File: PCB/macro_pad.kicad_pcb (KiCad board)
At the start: 2 copper layers, 112.3 x 92.7 mm, 57 parts, among them J1 OLED, J2 SWD, SW1 SW_Push_45deg, SW10 SW_Push_45deg, SW11 SW_Push_45deg, SW12 SW_Push_45deg, SW13 SW_Push_45deg, SW14 SW_Push_45deg, SW15 SW_Push_45deg, SW16 SW_Push_45deg, SW17 RotaryEncoder_Switch, SW18 RotaryEncoder_Switch, SW2 SW_Push_45deg, SW3 SW_Push_45deg, SW4 SW_Push_45deg, SW5 SW_Push_45deg, SW6 SW_Push_45deg, SW7 SW_Push_45deg, SW8 SW_Push_45deg, SW9 SW_Push_45deg

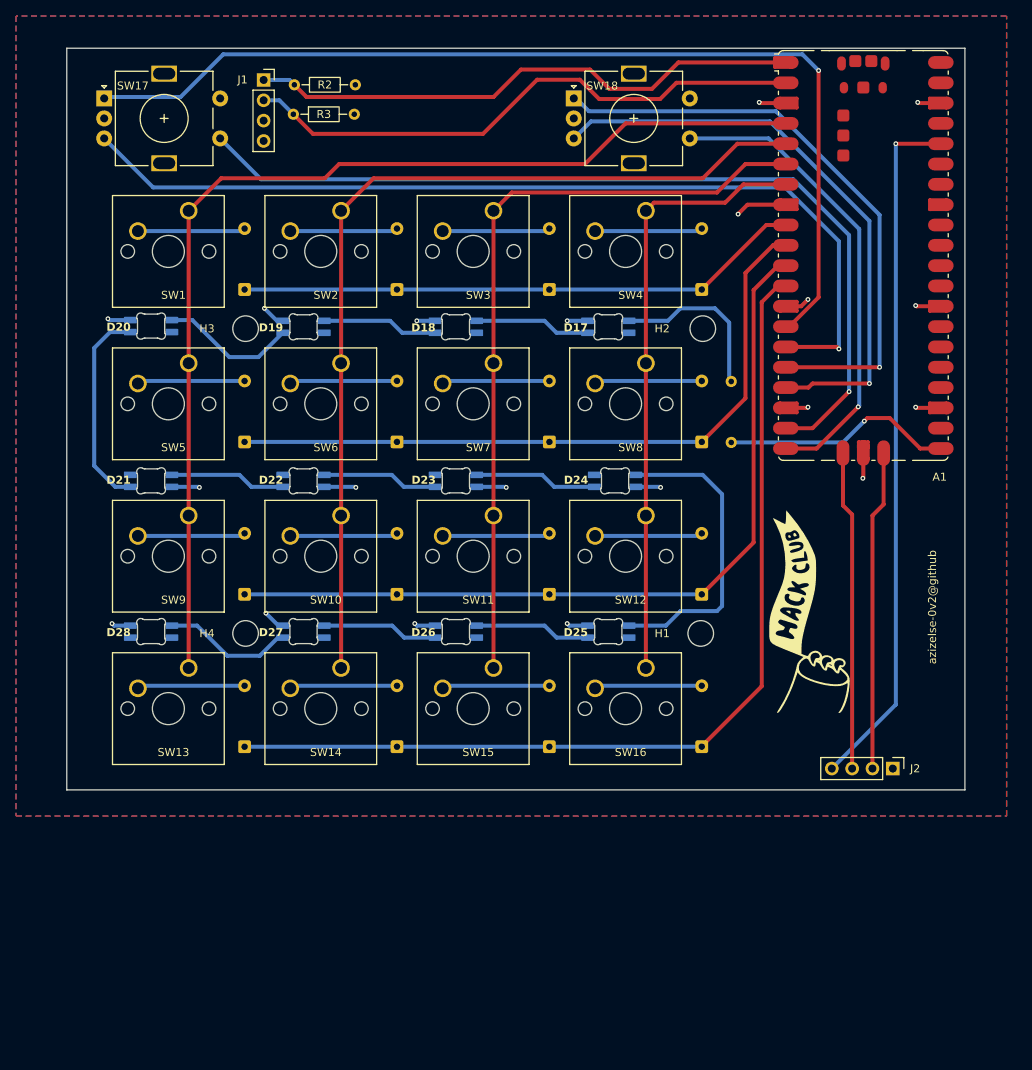
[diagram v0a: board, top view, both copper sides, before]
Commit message: Followed guidelines on schem
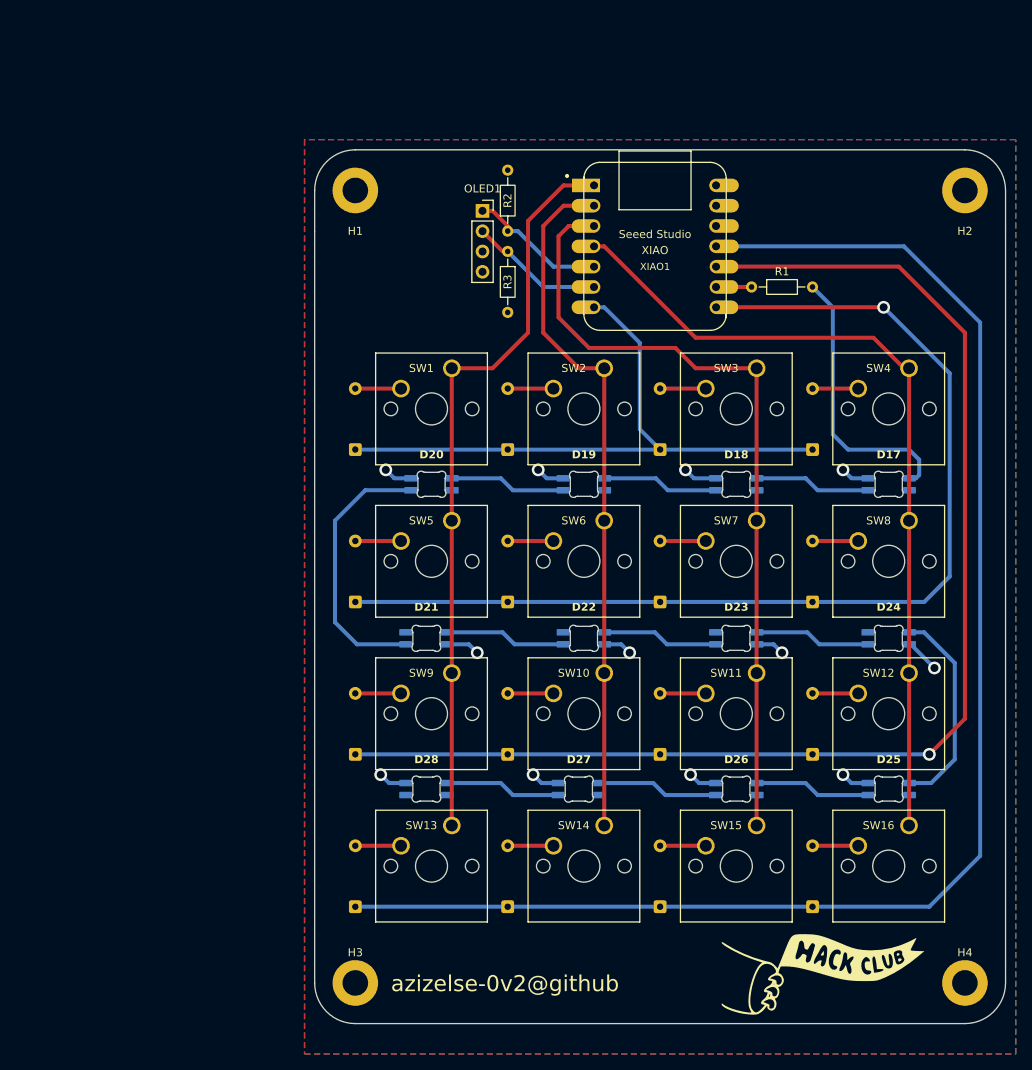
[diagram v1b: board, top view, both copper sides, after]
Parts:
- removed A1: RaspberryPi_Pico, Module:RaspberryPi_Pico_SMD
- removed J1: OLED, Connector_PinSocket_2.54mm:PinSocket_1x04_P2.54mm_Vertical
- removed J2: SWD, Connector_PinHeader_2.54mm:PinHeader_1x04_P2.54mm_Vertical
- removed SW17, SW18: RotaryEncoder_Switch, RotaryEncoder_Alps_EC11E-Switch_Vertical_H20mm:RotaryEncoder_Alps_EC11E-Switch_Vertical_H20mm
- added OLED1: OLED, Connector_PinSocket_2.54mm:PinSocket_1x04_P2.54mm_Vertical, F.Cu at (100.5, 60.6)
- added XIAO1: MOUDLE-SEEEDUINO-XIAO, XIAO_RP2040:XIAO_RP2040, F.Cu at (122.1, 65.0)
- H1, H2, H3, H4: value MountingHole -> MountingHole_Pad; footprint MountingHole:MountingHole_3.2mm_M3 -> MountingHole:MountingHole_3.2mm_M3_ISO7380_Pad
- R1: moved to F.Cu
- moved H4 100.0 mm to (160.8, 157.1)
- moved H3 82.9 mm to (84.6, 157.1)
- moved H1 70.2 mm to (84.6, 58.0)
- moved G*** 45.4 mm to (143.1, 155.9), turned to 0 degrees
- moved D20 40.2 mm to (94.2, 94.8)
- moved D17 40.2 mm to (151.3, 94.8)
- moved D19 40.2 mm to (113.2, 94.8)
- moved D22 40.2 mm to (113.2, 113.9)
- moved D25 40.2 mm to (151.3, 132.9)
- moved D18 40.2 mm to (132.3, 94.8)
- moved D23 40.2 mm to (132.3, 113.9)
- moved D26 40.2 mm to (132.3, 132.9)
- moved D21 39.6 mm to (93.5, 113.9)
- moved D27 39.6 mm to (112.6, 132.9)
- moved D28 39.6 mm to (93.5, 132.9)
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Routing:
- net /VlEncA: track 126.4 -> 0.00 mm, vias 1 -> 0
- net /VlEncB: track 117.4 -> 0.00 mm, vias 1 -> 0
- net /EncB1: track 113.0 -> 0.00 mm, vias 1 -> 0
- net +3V3: track 87.0 -> 0.00 mm, vias 1 -> 0
- net /BrEncA: track 75.0 -> 0.00 mm, vias 1 -> 0
- net /BrEncB: track 74.0 -> 0.00 mm, vias 1 -> 0
- net row3: track 119.7 -> 184.4 mm
- net /EncB2: track 59.4 -> 0.00 mm, vias 1 -> 0
- net row2: track 103.2 -> 160.8 mm, vias 0 -> 1
- net /SCL: track 71.7 -> 16.8 mm
- net /SDA: track 69.9 -> 17.2 mm
- net row1: track 87.0 -> 133.6 mm, vias 0 -> 1
- net column0: track 136.3 -> 92.6 mm
- net /SWDIO: track 40.9 -> 0.00 mm
- net /SWCLK: track 40.7 -> 0.00 mm
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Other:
- board size 112.3 x 92.7 mm -> 86.4 x 109.2 mm
